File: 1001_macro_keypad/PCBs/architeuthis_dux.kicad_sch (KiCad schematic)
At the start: 19 parts, among them J1 ePaperModule, J2 RotaryModule_01, J3 RotaryModule_02, SW01 MX_SW, SW10 MX_SW, SW11 MX_SW, SW12 MX_SW, SW13 MX_SW, SW14 MX_SW, SW2 MX_SW, SW3 MX_SW, SW4 MX_SW, SW5 MX_SW, SW6 MX_SW, SW7 MX_SW, SW8 MX_SW, SW9 MX_SW, U1 Pico

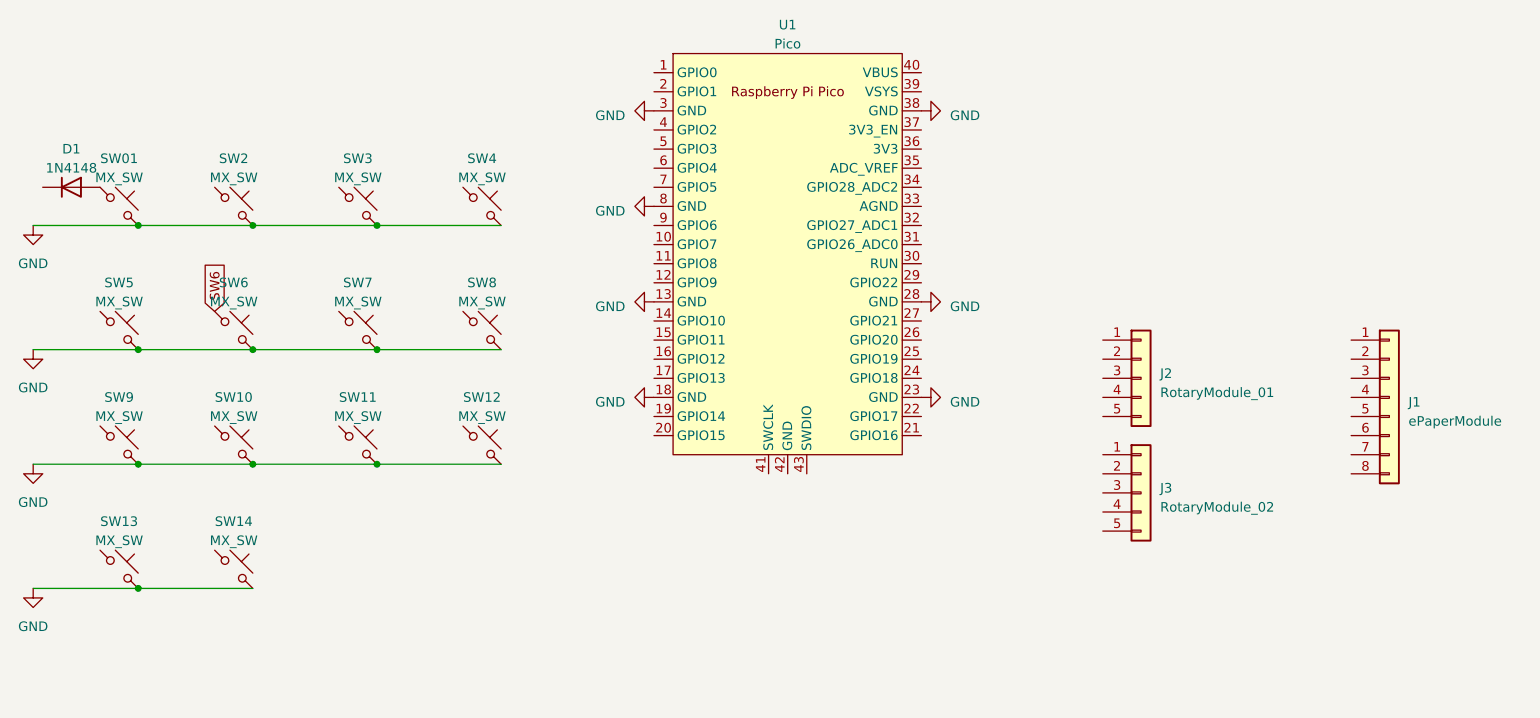
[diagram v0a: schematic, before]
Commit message: 배션중
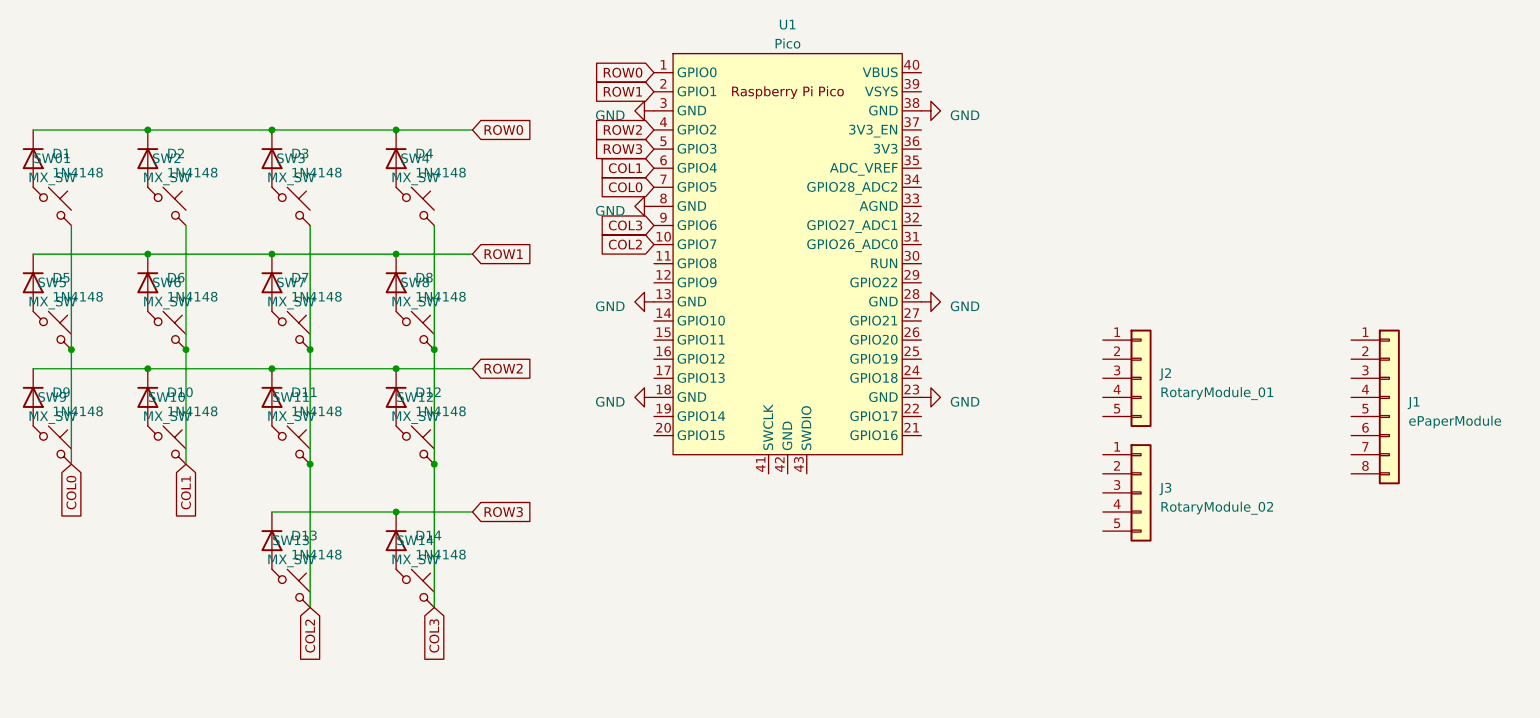
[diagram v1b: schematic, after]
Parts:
- added D10, D11, D12, D13, D14, D2, D3, D4, D5, D6, D7, D8, D9: 1N4148, Diode_THT:D_DO-35_SOD27_P7.62mm_Horizontal, symbol Diode:1N4148
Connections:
- net GND: no longer SW01.2, SW10.2, SW11.2, SW12.2, SW13.2, SW14.2, SW2.2, SW3.2, SW4.2, SW5.2, SW6.2, SW7.2, SW8.2, SW9.2
- net at SW3.1: now also D3.2 (A)
- net at SW8.1: now also D8.2 (A)
- net at SW11.1: now also D11.2 (A)
- net at SW2.1: now also D2.2 (A)
- net at SW14.1: now also D14.2 (A)
- net at SW13.1: now also D13.2 (A)
- net at SW9.1: now also D9.2 (A)
- net at SW5.1: now also D5.2 (A)
- net ROW0: now reaches D1.1 (K)
- net ROW0: now also U1.1 (GPIO0), D2.1 (K), D3.1 (K), D4.1 (K)
- net COL2: now reaches U1.10 (GPIO7)
- net COL2: now also SW11.2, SW13.2, SW3.2, SW7.2
- net ROW1: now reaches U1.2 (GPIO1)
- net ROW1: now also D5.1 (K), D6.1 (K), D7.1 (K), D8.1 (K)
- net ROW2: now reaches U1.4 (GPIO2)
- net ROW2: now also D10.1 (K), D11.1 (K), D12.1 (K), D9.1 (K)
- net ROW3: now reaches U1.5 (GPIO3)
- net ROW3: now also D13.1 (K), D14.1 (K)
- net COL1: now reaches U1.6 (GPIO4)
- net COL1: now also SW10.2, SW2.2, SW6.2
- net COL0: now reaches U1.7 (GPIO5)
- net COL0: now also SW01.2, SW5.2, SW9.2
- net COL3: now reaches U1.9 (GPIO6)
- net COL3: now also SW12.2, SW14.2, SW4.2, SW8.2
- net at SW7.1: now also D7.2 (A)
- net at SW12.1: now also D12.2 (A)
- net at SW10.1: now also D10.2 (A)
- net at SW4.1: now also D4.2 (A)
- net SW6: no longer names the net of SW6.1
- net SW6: now also D6.2 (A)
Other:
- moved on the sheet: D1, SW01, SW10, SW11, SW12, SW13, SW14, SW2, SW3, SW4, SW5, SW6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

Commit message: 재배선
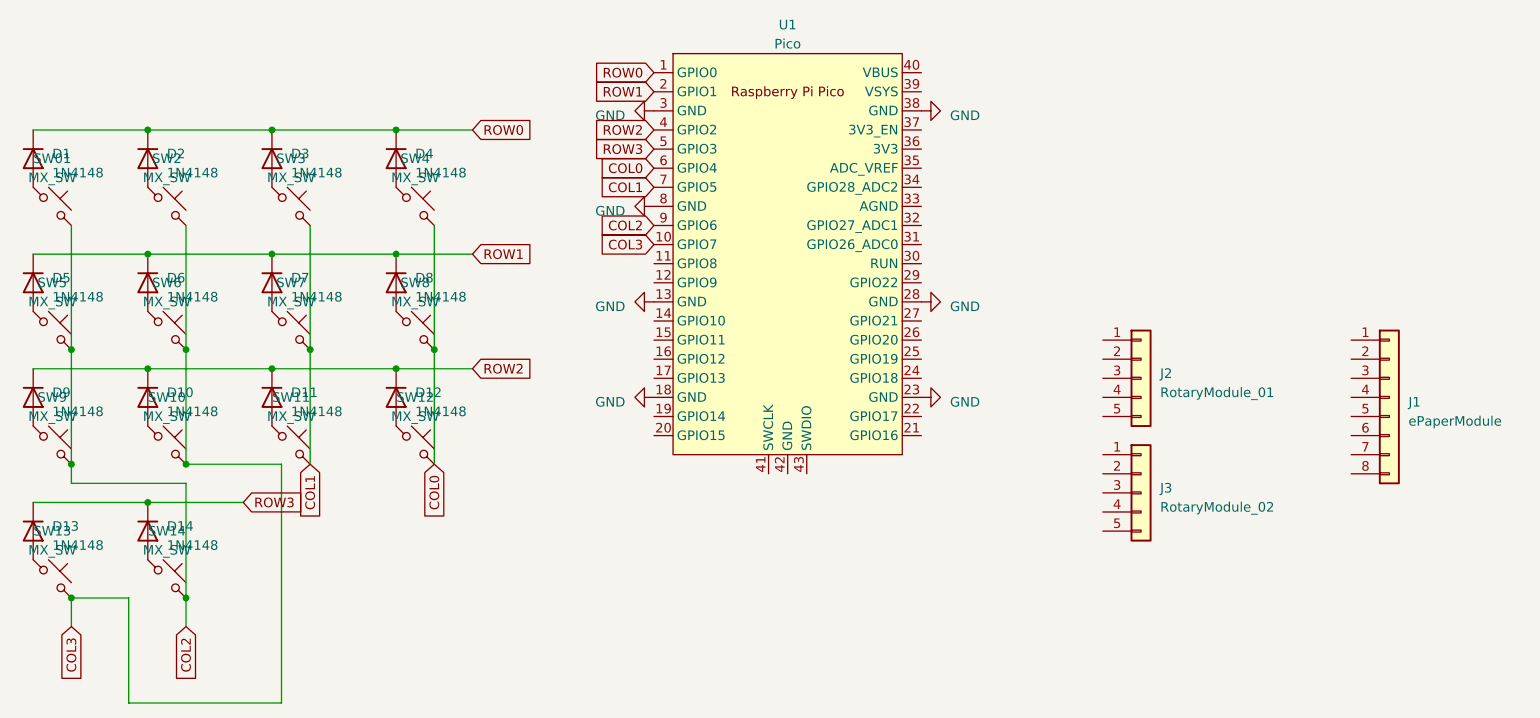
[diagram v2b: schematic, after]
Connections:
- net COL0: now also SW12.2, SW4.2, SW8.2, U1.6 (GPIO4); no longer SW01.2, SW5.2, SW9.2, U1.7 (GPIO5)
- net COL1: now also SW11.2, SW3.2, SW7.2, U1.7 (GPIO5); no longer SW10.2, SW2.2, SW6.2, U1.6 (GPIO4)
- net COL2: now also SW01.2, SW14.2, SW5.2, SW9.2, U1.9 (GPIO6); no longer SW11.2, SW13.2, SW3.2, SW7.2, U1.10 (GPIO7)
- net COL3: now also SW10.2, SW13.2, SW2.2, SW6.2, U1.10 (GPIO7); no longer SW12.2, SW14.2, SW4.2, SW8.2, U1.9 (GPIO6)
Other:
- moved on the sheet: D13, D14, SW13, SW14
